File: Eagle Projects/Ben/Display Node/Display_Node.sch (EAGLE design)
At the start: 54 parts, among them Q1 16MHz, Q3 16MHz, Q4 16MHz, Q5 16MHz, Q6 2N7002, Q7 2N7002, U1 ATMEGA328P_TQFP, U2 MCP2551, X1 5566-6, X2 5566-6

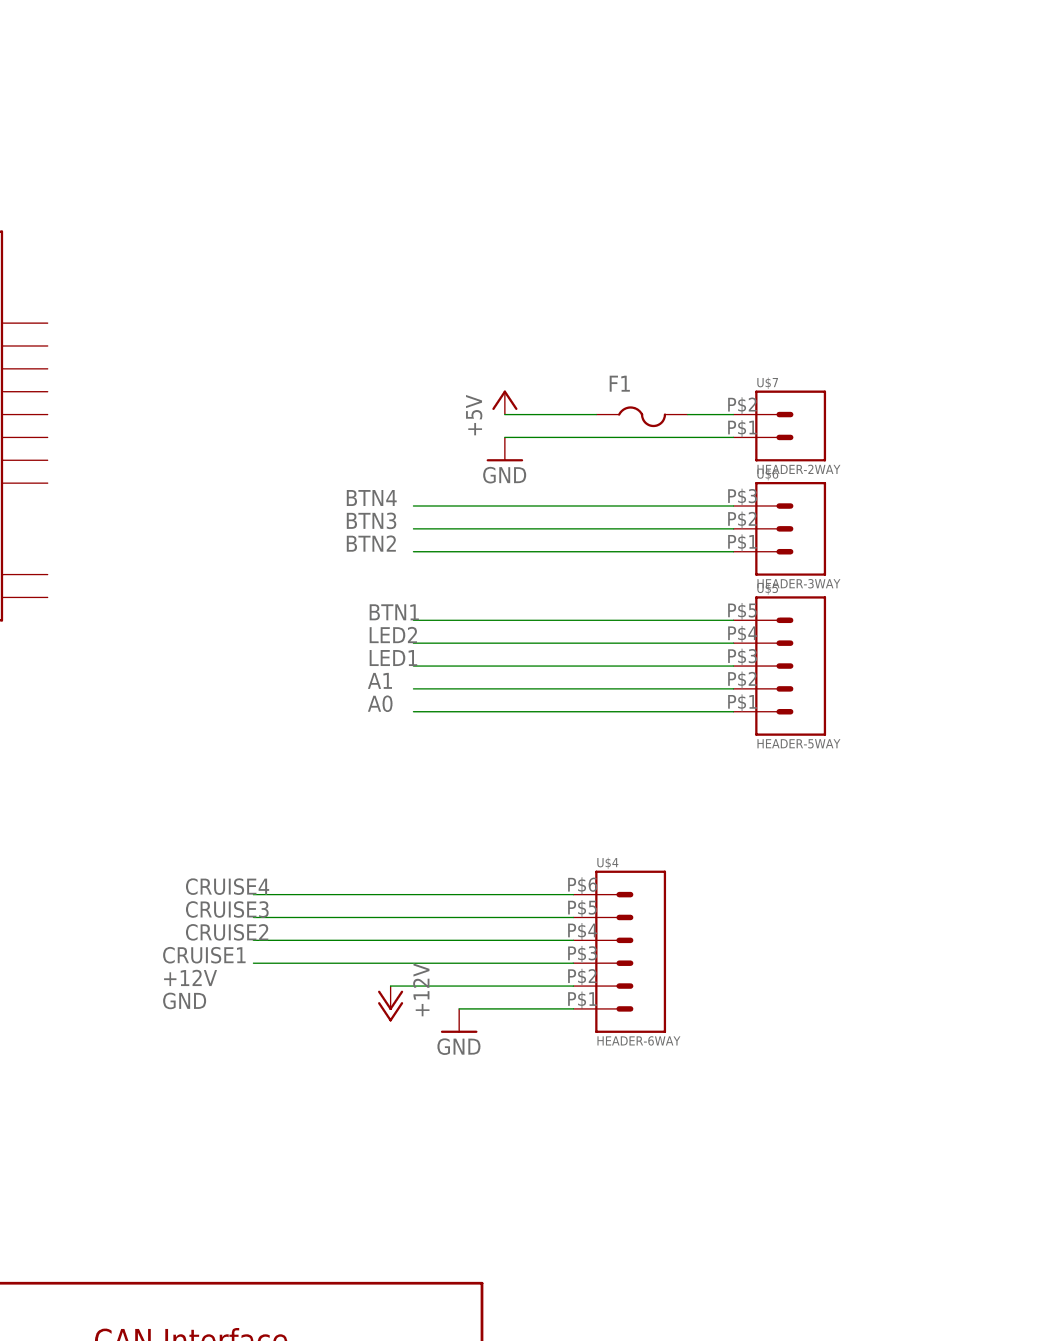
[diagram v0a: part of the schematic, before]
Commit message: Working On Protection
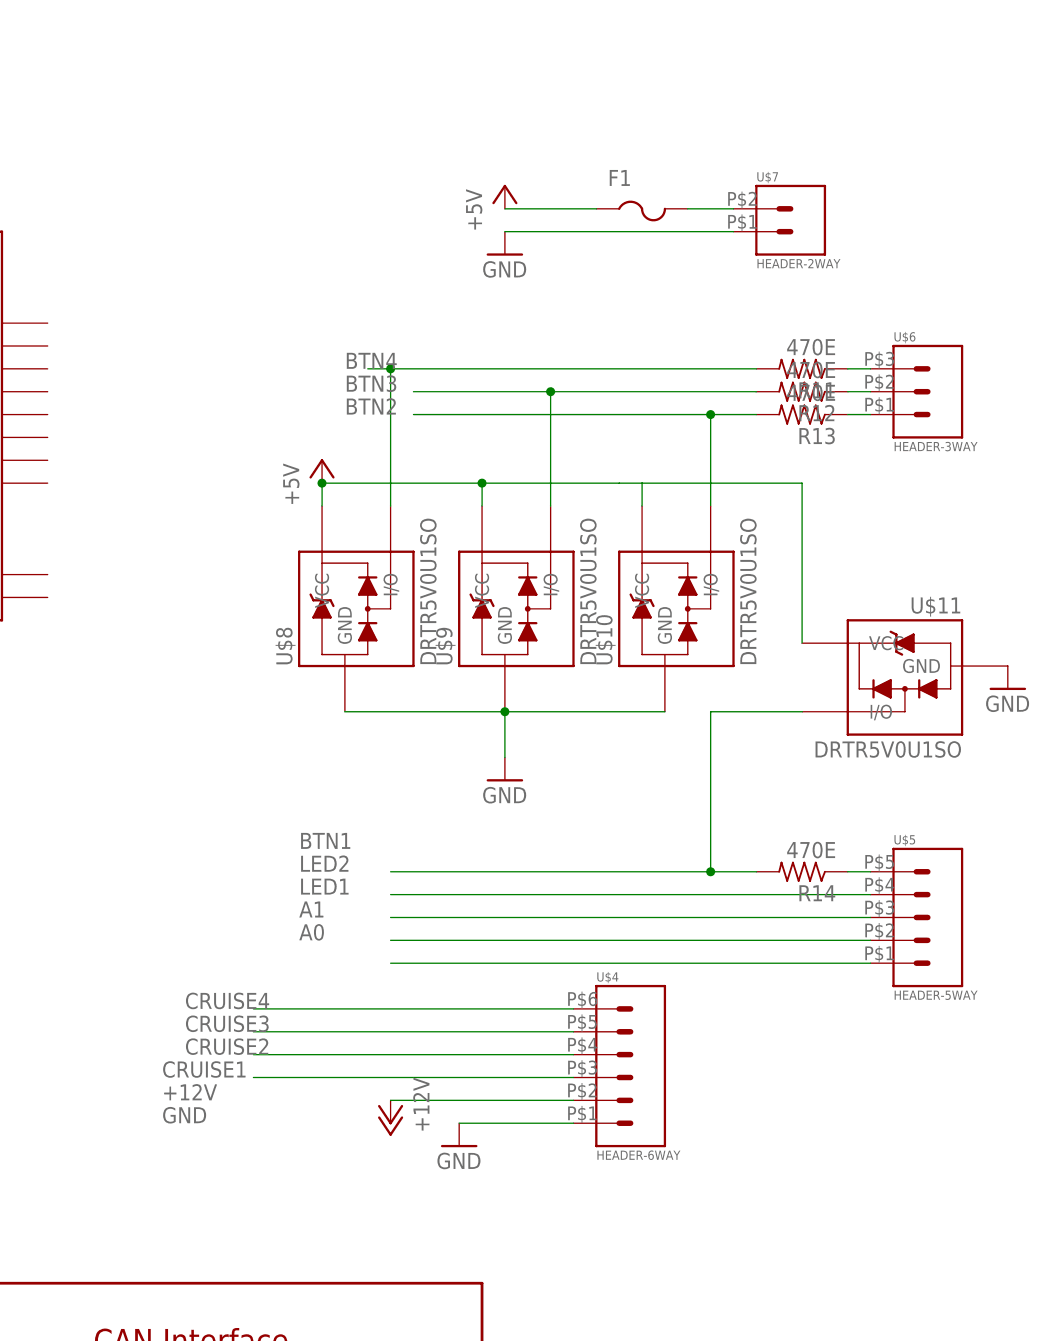
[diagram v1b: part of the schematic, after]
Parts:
- added R11, R12, R13, R14: 470E, resistor:R-US_R0805
- added U$10, U$11, U$8, U$9: DRTR5V0U1SO, RobThePyro:DRTR5V0U1SO
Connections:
- new net N$18: R11.1, U$6.P$3
- new net N$19: R12.1, U$6.P$2
- new net N$20: R13.1, U$6.P$1
- new net N$21: R14.1, U$5.P$5
- net +5V: now also U$10.VCC, U$11.VCC, U$8.VCC, U$9.VCC
- net BTN1: now also R14.2, U$11.I/O; no longer U$5.P$5
- net BTN2: now also R13.2, U$10.I/O; no longer U$6.P$1
- net BTN3: now also R12.2, U$9.I/O; no longer U$6.P$2
- net BTN4: now also R11.2, U$8.I/O; no longer U$6.P$3
- net GND: now also U$10.GND, U$11.GND, U$8.GND, U$9.GND
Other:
- moved on the sheet: F1, U$4, U$5, U$6, U$7
